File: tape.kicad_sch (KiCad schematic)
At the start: 7 parts, among them J9 PJ-320D

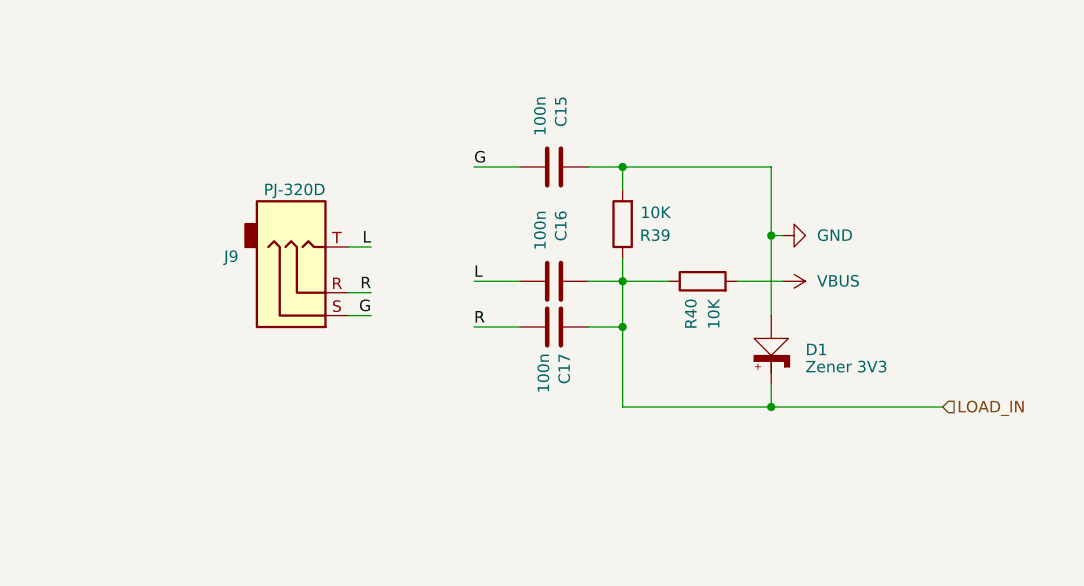
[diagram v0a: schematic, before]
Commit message: Rev 1.05 WIP
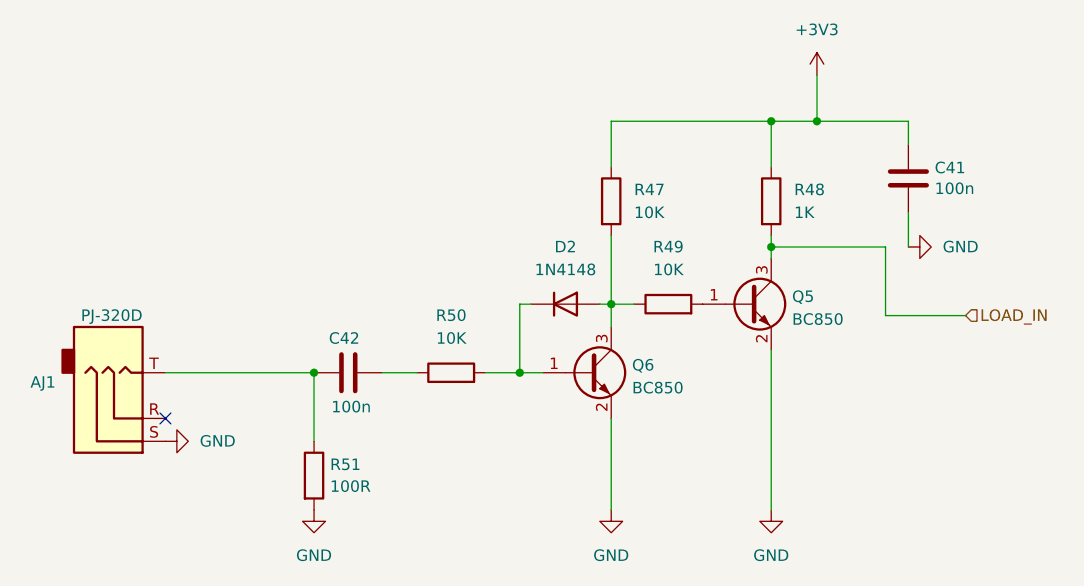
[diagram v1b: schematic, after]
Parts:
- removed C15, C16, C17: 100n, FRANK:Capacitor (0805), symbol Device:C
- removed D1: Zener 3V3, FRANK:Diode (0805), symbol PCM_Nuova-Elettronica-Diodes:Zener
- removed J9: PJ-320D, FRANK:Jack (3.5mm, PJ-320D), symbol FRANK:AudioJack_3.5mm
- removed R39, R40: 10K, FRANK:Resistor (0805), symbol Device:R
- added AJ1: PJ-320D, FRANK:Jack (3.5mm, PJ-320D), symbol FRANK:AudioJack_3.5mm
- added C41, C42: 100n, FRANK:Capacitor (0603), symbol Device:C
- added D2: 1N4148, FRANK:Diode (SOD-323), symbol Device:D
- added Q5, Q6: BC850, FRANK:SOT-23, symbol Transistor_BJT:BC850
- added R47, R49, R50: 10K, FRANK:Resistor (0603), symbol Device:R
- added R48: 1K, FRANK:Resistor (0603), symbol Device:R
- added R51: 100R, FRANK:Resistor (0603), symbol Device:R
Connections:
- net GND: now also AJ1.S, C41.2, Q5.2 (E), Q6.2 (E), R51.2
- net LOAD_IN: now also Q5.3 (C), R48.2
- new net: D2.2 (A), Q6.3 (C), R47.2, R49.1
- new net: D2.1 (K), Q6.1 (B), R50.2
- new net: AJ1.T, C42.1, R51.1
- new net: C42.2, R50.1
- new net: Q5.1 (B), R49.2
- new net +3V3: C41.1, R47.1, R48.1
- no-connect marks 0 -> 1
